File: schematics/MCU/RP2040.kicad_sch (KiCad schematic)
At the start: 37 parts, among them J2 TC2030, Q1 2N7002, SW1 SW_Push, SW2 SW_Push, U1 W25Q128JVS, U2 XC6206PxxxMR-Regulator_Linear, U3 RP2040, Y1 12MHz

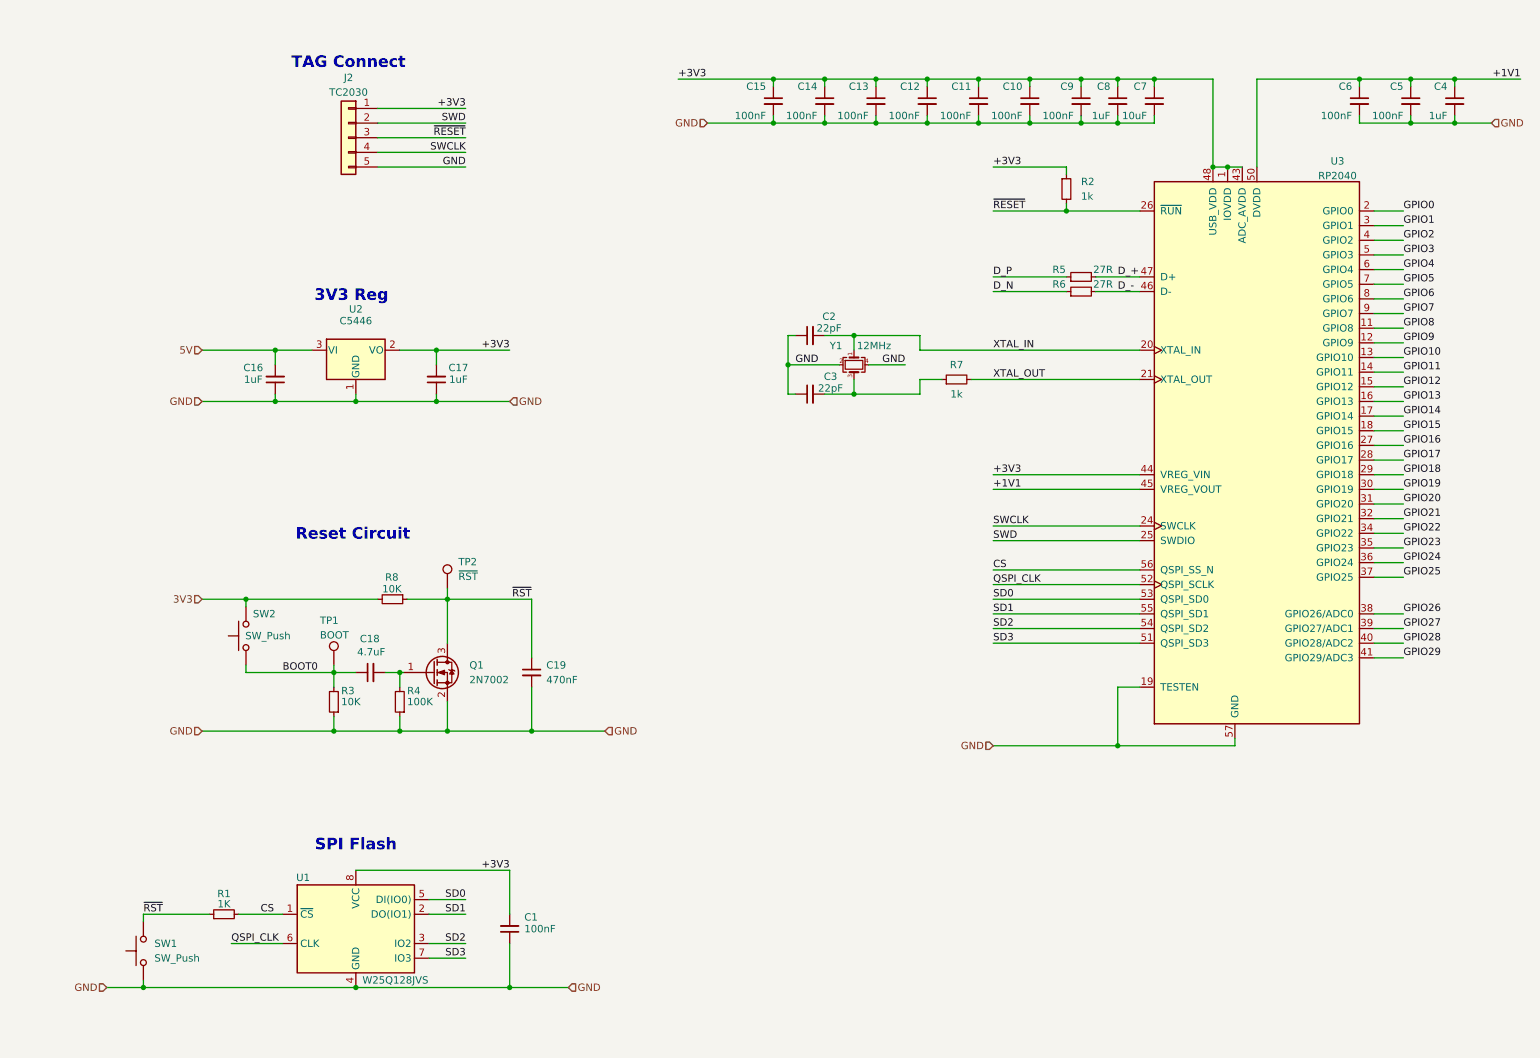
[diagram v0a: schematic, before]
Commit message: Minor updates to STM32, refactor RP2040
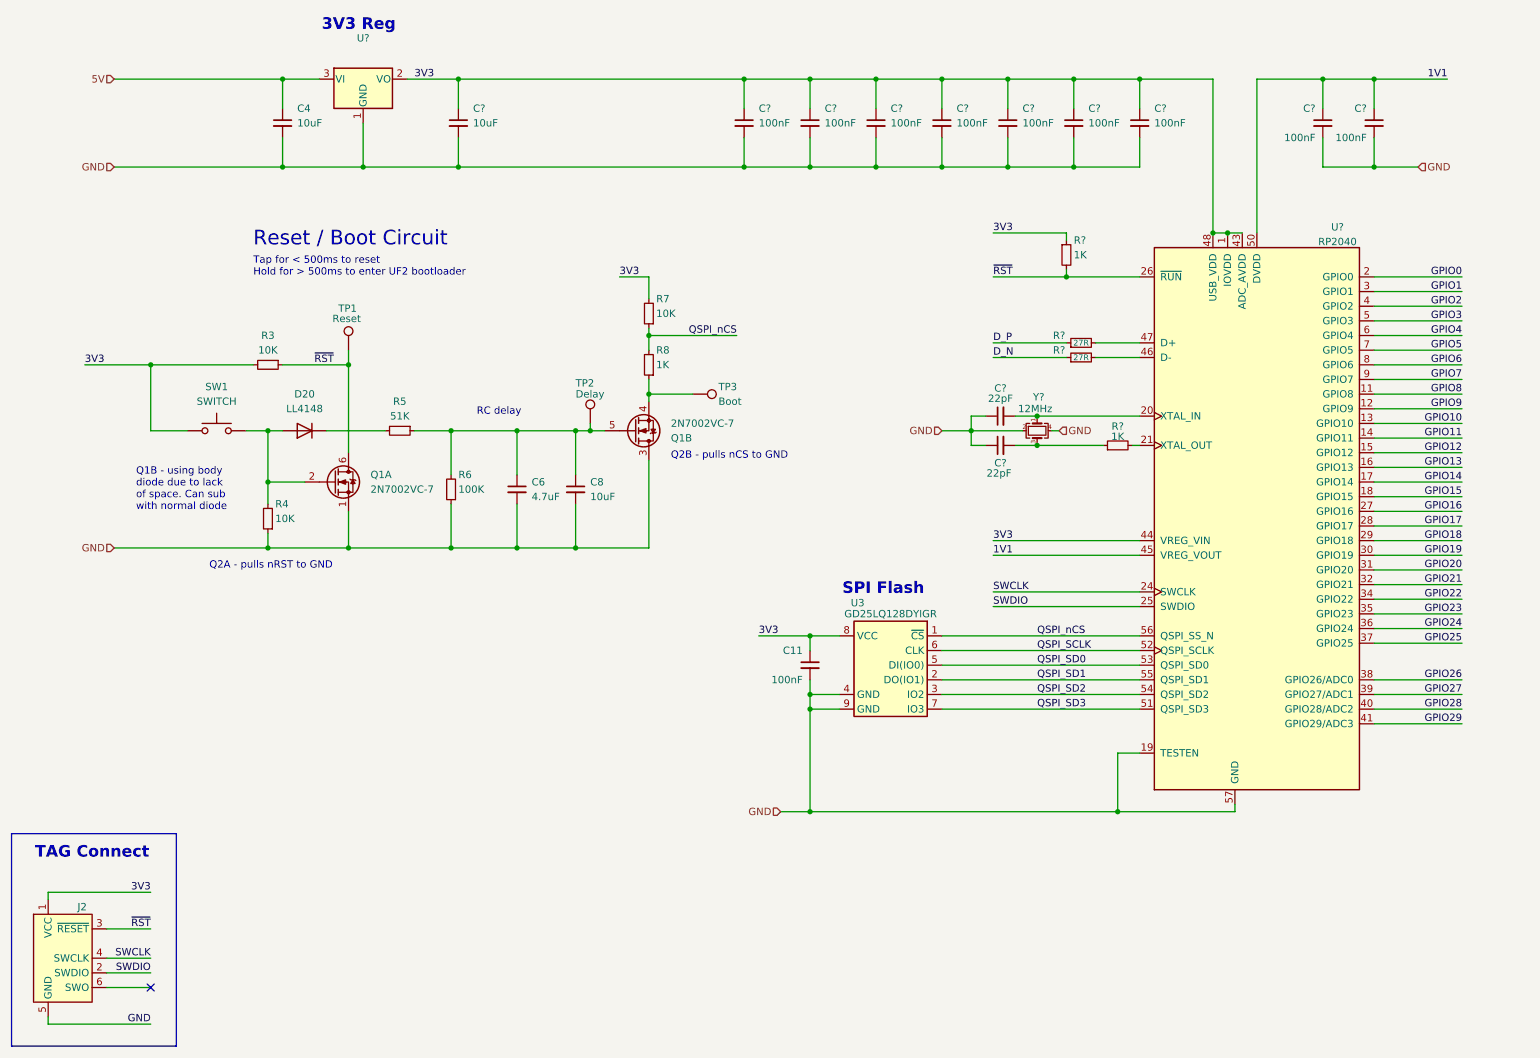
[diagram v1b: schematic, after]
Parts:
- removed C1: 100nF, Capacitor_SMD:C_0402_1005Metric, symbol Device:C_Small
- removed C16, C17: 1uF, Capacitor_SMD:C_0402_1005Metric, symbol Device:C_Small
- removed C18: 4.7uF, Capacitor_SMD:C_0603_1608Metric, symbol Device:C_Small
- removed C19: 470nF, Capacitor_SMD:C_0603_1608Metric, symbol Device:C_Small
- removed J2: TC2030, Connector:Tag-Connect_TC2030-IDC-NL_2x03_P1.27mm_Vertical, symbol Connector_Generic:Conn_01x05
- removed Q1: 2N7002, Package_TO_SOT_SMD:SOT-23, symbol Transistor_FET:2N7002
- removed R1: 1K, Resistor_SMD:R_0402_1005Metric, symbol Device:R_Small
- removed SW2: SW_Push, symbol Switch:SW_Push
- removed U1: W25Q128JVS, Package_SO:SOIC-8_5.23x5.23mm_P1.27mm, symbol Memory_Flash:W25Q128JVS
- added C11: 100nF, Capacitor_SMD:C_0402_1005Metric, symbol Device:C_Small
- added C6: 4.7uF, Capacitor_SMD:C_0805_2012Metric, symbol Device:C_Small
- added D20: LL4148, Diode_SMD:D_MiniMELF, symbol Diode:LL4148
- added J2: Conn_ARM_SWD_TagConnect_TC2030-NL, Connector:Tag-Connect_TC2030-IDC-NL_2x03_P1.27mm_Vertical, symbol Connector:Conn_ARM_SWD_TagConnect_TC2030-NL
- added Q1: 2N7002VC-7, Package_TO_SOT_SMD:SOT-363_SC-70-6, symbol Transistor_FET:FDG6335N
- added R5: 51K, Resistor_SMD:R_0402_1005Metric, symbol Device:R_Small
- added R6: 100K, Resistor_SMD:R_0402_1005Metric, symbol Device:R_Small
- added R7: 10K, Resistor_SMD:R_0402_1005Metric, symbol Device:R_Small
- added TP3: Boot, TestPoint:TestPoint_Pad_D1.0mm, symbol Connector:TestPoint
- added U3: GD25LQ128DYIGR, Package_SON:WSON-8-1EP_6x5mm_P1.27mm_EP3.4x4mm, symbol josh-memory:W25Q128JVSIQ
- C4, C8: value 1uF -> 10uF; LCSC C52923 -> (none); MPN (none) -> C0805C106K3PAC7800; Manufacturer (none) -> KEMET; Price (none) -> $0.43; Rating (none) -> CAP CER 10UF 25V X5R 0805; Supplier (none) -> Digikey; Supplier PN (none) -> 399-11939-1-ND
- C?: renamed from C12; LCSC C1525 -> (none); MPN (none) -> C0402C104K3RAC7867; Manufacturer (none) -> KEMET; Price (none) -> $0.33; Rating (none) -> CAP CER 0.1UF 25V X7R 0402; Supplier (none) -> Digikey; Supplier PN (none) -> 399-14148-1-ND
- C?: renamed from C7; LCSC C15525 -> (none); MPN (none) -> C0805C106K3PAC7800; Manufacturer (none) -> KEMET; Price (none) -> $0.43; Rating (none) -> CAP CER 10UF 25V X5R 0805; Supplier (none) -> Digikey; Supplier PN (none) -> 399-11939-1-ND
- C?: renamed from C15; LCSC C1525 -> (none); MPN (none) -> C0402C104K3RAC7867; Manufacturer (none) -> KEMET; Price (none) -> $0.33; Rating (none) -> CAP CER 0.1UF 25V X7R 0402; Supplier (none) -> Digikey; Supplier PN (none) -> 399-14148-1-ND
- C?: renamed from C14; LCSC C1525 -> (none); MPN (none) -> C0402C104K3RAC7867; Manufacturer (none) -> KEMET; Price (none) -> $0.33; Rating (none) -> CAP CER 0.1UF 25V X7R 0402; Supplier (none) -> Digikey; Supplier PN (none) -> 399-14148-1-ND
- C?: renamed from C11; LCSC C1525 -> (none); MPN (none) -> C0402C104K3RAC7867; Manufacturer (none) -> KEMET; Price (none) -> $0.33; Rating (none) -> CAP CER 0.1UF 25V X7R 0402; Supplier (none) -> Digikey; Supplier PN (none) -> 399-14148-1-ND
- C?: renamed from C10; LCSC C1525 -> (none); MPN (none) -> C0402C104K3RAC7867; Manufacturer (none) -> KEMET; Price (none) -> $0.33; Rating (none) -> CAP CER 0.1UF 25V X7R 0402; Supplier (none) -> Digikey; Supplier PN (none) -> 399-14148-1-ND
- C?: renamed from C2; LCSC C1555 -> (none); MPN (none) -> C0402C220J4GAC7867; Manufacturer (none) -> KEMET; Price (none) -> 0.16; Rating (none) -> CAP CER 22PF 16V C0G/NP0 0402; Supplier (none) -> Digikey; Supplier PN (none) -> 399-C0402C220J4GAC7867CT-ND
- C?: renamed from C13; LCSC C1525 -> (none); MPN (none) -> C0402C104K3RAC7867; Manufacturer (none) -> KEMET; Price (none) -> $0.33; Rating (none) -> CAP CER 0.1UF 25V X7R 0402; Supplier (none) -> Digikey; Supplier PN (none) -> 399-14148-1-ND
- C?: renamed from C5; LCSC C1525 -> (none); MPN (none) -> C0402C104K3RAC7867; Manufacturer (none) -> KEMET; Price (none) -> $0.33; Rating (none) -> CAP CER 0.1UF 25V X7R 0402; Supplier (none) -> Digikey; Supplier PN (none) -> 399-14148-1-ND
- C?: renamed from C3; LCSC C1555 -> (none); MPN (none) -> C0402C220J4GAC7867; Manufacturer (none) -> KEMET; Price (none) -> 0.16; Rating (none) -> CAP CER 22PF 16V C0G/NP0 0402; Supplier (none) -> Digikey; Supplier PN (none) -> 399-C0402C220J4GAC7867CT-ND
- C?: renamed from C9; LCSC C1525 -> (none); MPN (none) -> C0402C104K3RAC7867; Manufacturer (none) -> KEMET; Price (none) -> $0.33; Rating (none) -> CAP CER 0.1UF 25V X7R 0402; Supplier (none) -> Digikey; Supplier PN (none) -> 399-14148-1-ND
- C?: renamed from C6; LCSC C1525 -> (none); MPN (none) -> C0402C104K3RAC7867; Manufacturer (none) -> KEMET; Price (none) -> $0.33; Rating (none) -> CAP CER 0.1UF 25V X7R 0402; Supplier (none) -> Digikey; Supplier PN (none) -> 399-14148-1-ND
- R3: footprint Resistor_SMD:R_0603_1608Metric -> Resistor_SMD:R_0402_1005Metric; MPN (none) -> RC0402FR-0710KL; Manufacturer (none) -> YAGEO; Price (none) -> $0.16; Rating (none) -> RES 10K OHM 1% 1/16W 0402; Supplier (none) -> Digikey; Supplier PN (none) -> 311-10.0KLRCT-ND
- R4: value 100K -> 10K; footprint Resistor_SMD:R_0603_1608Metric -> Resistor_SMD:R_0402_1005Metric; MPN (none) -> RC0402FR-0710KL; Manufacturer (none) -> YAGEO; Price (none) -> $0.16; Rating (none) -> RES 10K OHM 1% 1/16W 0402; Supplier (none) -> Digikey; Supplier PN (none) -> 311-10.0KLRCT-ND
- R8: value 10K -> 1K; footprint Resistor_SMD:R_0603_1608Metric -> Resistor_SMD:R_0402_1005Metric; MPN (none) -> RC0402FR-071KL; Manufacturer (none) -> YAGEO; Price (none) -> $0.16; Rating (none) -> RES 1K OHM 1% 1/16W 0402; Supplier (none) -> Digikey; Supplier PN (none) -> 311-1.00KLRCT-ND
- R?: renamed from R2; value 1k -> 1K; LCSC C11702 -> (none); MPN (none) -> RC0402FR-071KL; Manufacturer (none) -> YAGEO; Price (none) -> $0.16; Rating (none) -> RES 1K OHM 1% 1/16W 0402; Supplier (none) -> Digikey; Supplier PN (none) -> 311-1.00KLRCT-ND
- R?: renamed from R5; footprint Resistor_SMD:R_0603_1608Metric -> Resistor_SMD:R_0402_1005Metric; LCSC C25190 -> (none); MPN (none) -> RC0402FR-0727RL; Manufacturer (none) -> YAGEO; Price (none) -> $0.16; Rating (none) -> RES 27 Ohms ±1% 0.063W, 1/16W Chip Resistor 0402 (1005 Metr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; Supplier (none) -> Digikey; Supplier PN (none) -> YAG3086CT-ND
- R?: renamed from R6; footprint Resistor_SMD:R_0603_1608Metric -> Resistor_SMD:R_0402_1005Metric; LCSC C25190 -> (none); MPN (none) -> RC0402FR-0727RL; Manufacturer (none) -> YAGEO; Price (none) -> $0.16; Rating (none) -> RES 27 Ohms ±1% 0.063W, 1/16W Chip Resistor 0402 (1005 Metr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; Supplier (none) -> Digikey; Supplier PN (none) -> YAG3086CT-ND
- R?: renamed from R7; value 1k -> 1K; LCSC C11702 -> (none); MPN (none) -> RC0402FR-071KL; Manufacturer (none) -> YAGEO; Price (none) -> $0.16; Rating (none) -> RES 1K OHM 1% 1/16W 0402; Supplier (none) -> Digikey; Supplier PN (none) -> 311-1.00KLRCT-ND
- SW1: value SW_Push -> SWITCH; footprint Connector_PinSocket_2.54mm:PinSocket_1x02_P2.54mm_Vertical -> (none); now in the parts list
- TP1: value BOOT -> Reset; footprint (none) -> TestPoint:TestPoint_Pad_D1.0mm
- TP2: value ~{RST} -> Delay; footprint (none) -> TestPoint:TestPoint_Pad_D1.0mm
- U?: renamed from U3; footprint Sleep-Lib:RP2040-QFN-56 -> Package_DFN_QFN:QFN-56-1EP_7x7mm_P0.4mm_EP3.2x3.2mm; LCSC C2040 -> (none); MPN (none) -> SC0914(13); Manufacturer (none) -> Raspberry Pi; Price (none) -> $1.11; Rating (none) -> IC MCU 32BIT EXT MEM 56QFN; Supplier (none) -> Digikey; Supplier PN (none) -> 2648-SC0914(13)CT-ND
- U?: renamed from U2; LCSC C5446 -> (none)
- Y?: renamed from Y1; footprint Crystal:Crystal_SMD_3225-4Pin_3.2x2.5mm -> Crystal_SMD_Abracon_ABM8G-4Pin_3.2x2.5mm; LCSC C9002 -> (none); MPN (none) -> ABM8-12.000MHZ-12-B1U-T; Manufacturer (none) -> Abracon LLC; Price (none) -> $0.67; Rating (none) -> CRYSTAL 12.0000MHZ 12PF SMD; Supplier (none) -> Digikey; Supplier PN (none) -> 535-14962-1-ND
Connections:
- net CS is gone; now on net QSPI_nCS: U?.56 (QSPI_SS_N)
- net ~{RESET} is gone; now on net ~{RST}: R?.2, U?.26 (~{RUN})
- net 5V: now also C4.1
- net DVDD: no longer C4.1
- net GND: now also C11.2, C6.2, J2.5 (GND), Q1.1 (S), Q1.3 (D), R6.1, U3.4 (GND), U3.9 (GND); no longer R3.1, SW1.1
- net IOVDD: now also R3.2, SW1.2, C11.1, J2.1 (VCC), R7.2, U3.8 (VCC); no longer C8.1
- net SWCLK: now also J2.4 (SWCLK)
- net ~{RST}: now also R3.1, TP1.1, J2.3 (~{RESET}), Q1.6 (D); no longer R8.1, SW1.2, TP2.1
- net at R4.2: now also SW1.1, D20.2 (A), Q1.2 (G)
- net 3V3 renamed QSPI_nCS
- net QSPI_nCS: now also R7.1, U3.1 (~{CS})
- removed net BOOT0: R3.2, TP1.1
- net D_+: no longer names the net of R?.2, U?.47 (D+)
- net D_-: no longer names the net of R?.2, U?.46 (D-)
- net QSPI_CLK renamed QSPI_SCLK
- net QSPI_SCLK: now also U3.6 (CLK)
- net SD0 renamed QSPI_SD0
- net QSPI_SD0: now also U3.5 (DI(IO0))
- net SD1 renamed QSPI_SD1
- net QSPI_SD1: now also U3.2 (DO(IO1))
- net SD2 renamed QSPI_SD2
- net QSPI_SD2: now also U3.3 (IO2)
- net SD3 renamed QSPI_SD3
- net QSPI_SD3: now also U3.7 (IO3)
- net SWD renamed SWDIO
- net SWDIO: now also J2.2 (SWDIO)
- net XTAL_IN: no longer names the net of C?.2, U?.20 (XTAL_IN), Y?.1
- net XTAL_OUT: no longer names the net of R?.2, U?.21 (XTAL_OUT)
- new net: Q1.4 (S), R8.1, TP3.1
- new net: C6.1, C8.1, Q1.5 (G), R5.1, R6.2, TP2.1
- new net: D20.1 (K), R5.2
- no-connect marks 0 -> 1
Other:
- note added: "Q1B - using body diode due to lack of space. Can sub with normal diode"
- note added: "Q2A - pulls nRST to GND"
- note added: "Q2B - pulls nCS to GND"
- note added: "RC delay"
- note added: "Reset / Boot Circuit"
- note added: "Tap for < 500ms to reset Hold for > 500ms to enter UF2 bootloader"
- note removed: "Reset Circuit"
- moved on the sheet: C?, R?, U?, Y?
